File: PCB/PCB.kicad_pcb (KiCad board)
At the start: 2 copper layers, 53 parts, among them J1 USB_C_Receptacle_USB2.0_14P, Q1 IRLML2060, SW1 SW_Push, SW2 SW_Push, U1 RP2040, U2 W25Q16JVSS, U4 NCP1117-3.3_SOT223, U5 USBLC6-2SC6, Y1 Crystal_GND24

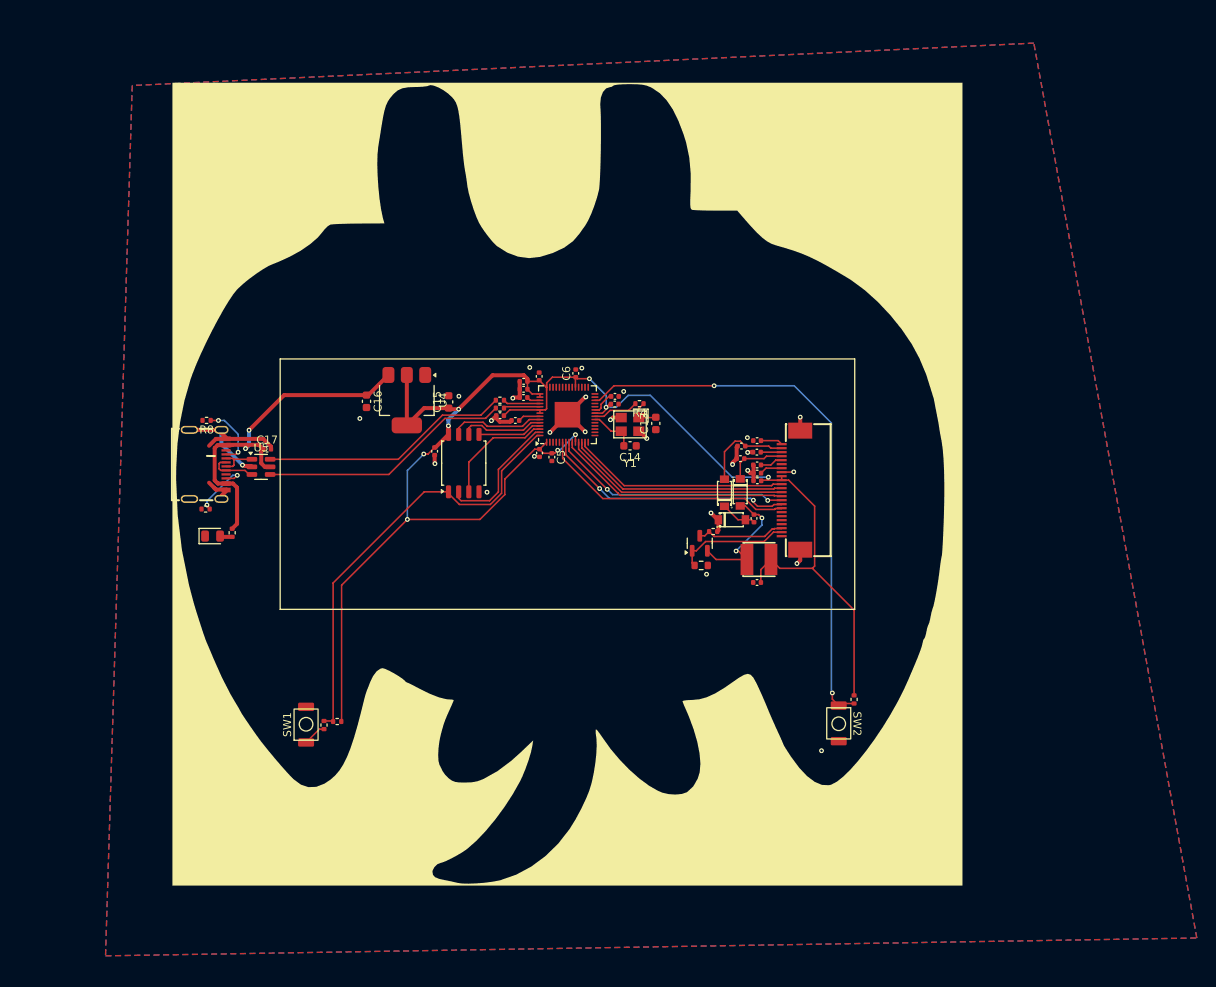
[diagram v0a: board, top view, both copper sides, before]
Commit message: commit beeg stuff(i forgor to commit for a while)
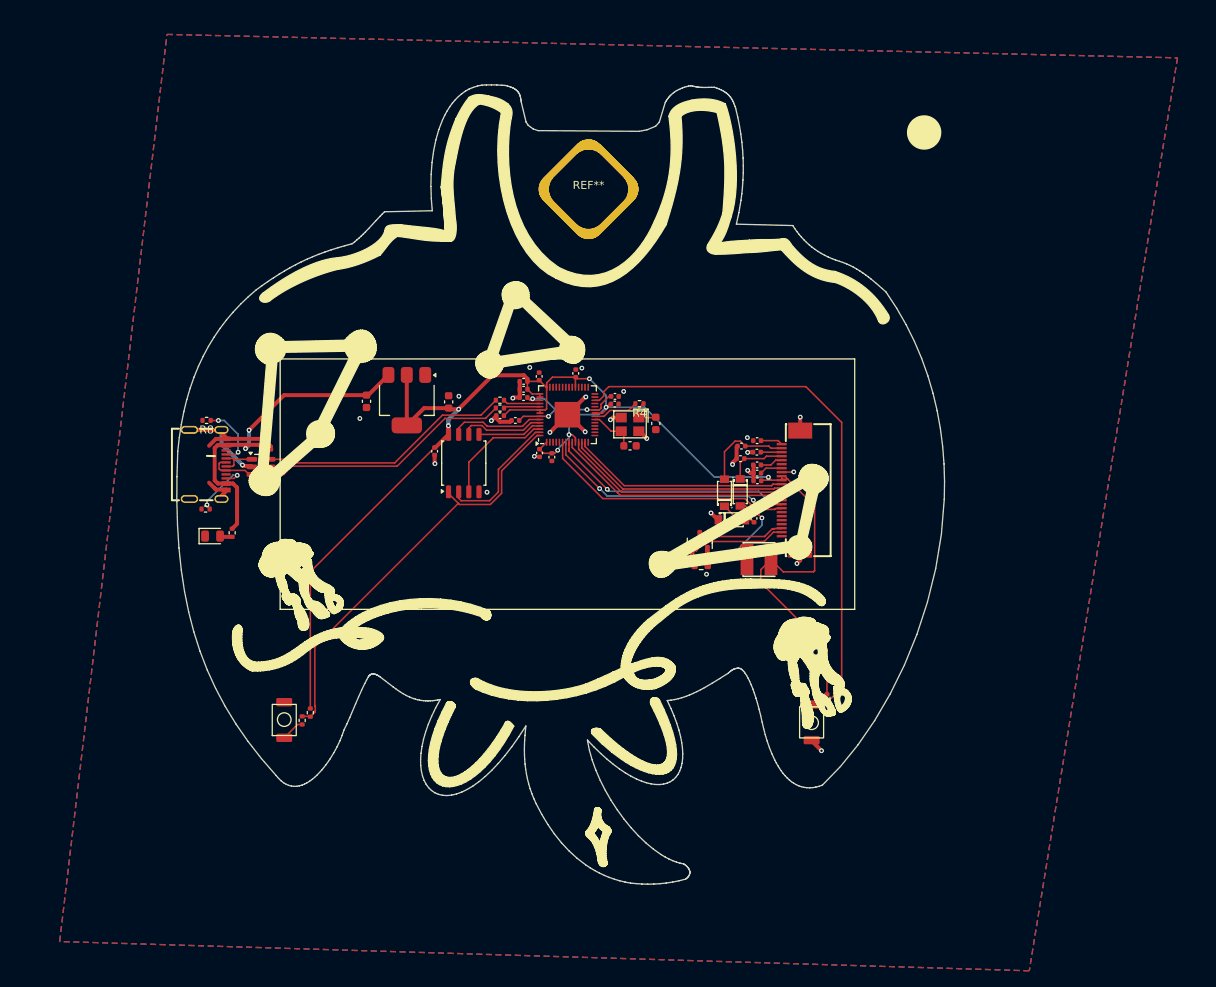
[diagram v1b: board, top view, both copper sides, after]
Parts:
- removed G***: LOGO, LOGO
- added REF**: Lanyard_hole2, Taranium-libs:Lanyard_hole2, F.Cu at (118.1, 34.1)
- moved R2 3.54 mm to (83.3, 99.6), turned to 90 degrees
- moved SW2 3.39 mm to (145.9, 100.8)
- moved R5 3.39 mm to (147.9, 97.8)
- moved R1 2.79 mm to (82.3, 100.5)
- moved SW1 2.79 mm to (80.0, 100.5)
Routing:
- net +3V3: track 198.6 -> 184.4 mm, vias 9 -> 7
- net +1V1: track 7.53 -> 18.4 mm, vias 0 -> 3
- net CS: track 55.1 -> 53.0 mm
- net GND: track 60.1 -> 61.9 mm
- net Net-(U1-RUN): track 70.0 -> 71.5 mm, vias 2 -> 0
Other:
- board outline added: 96 x 99.9 mm

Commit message: bleh
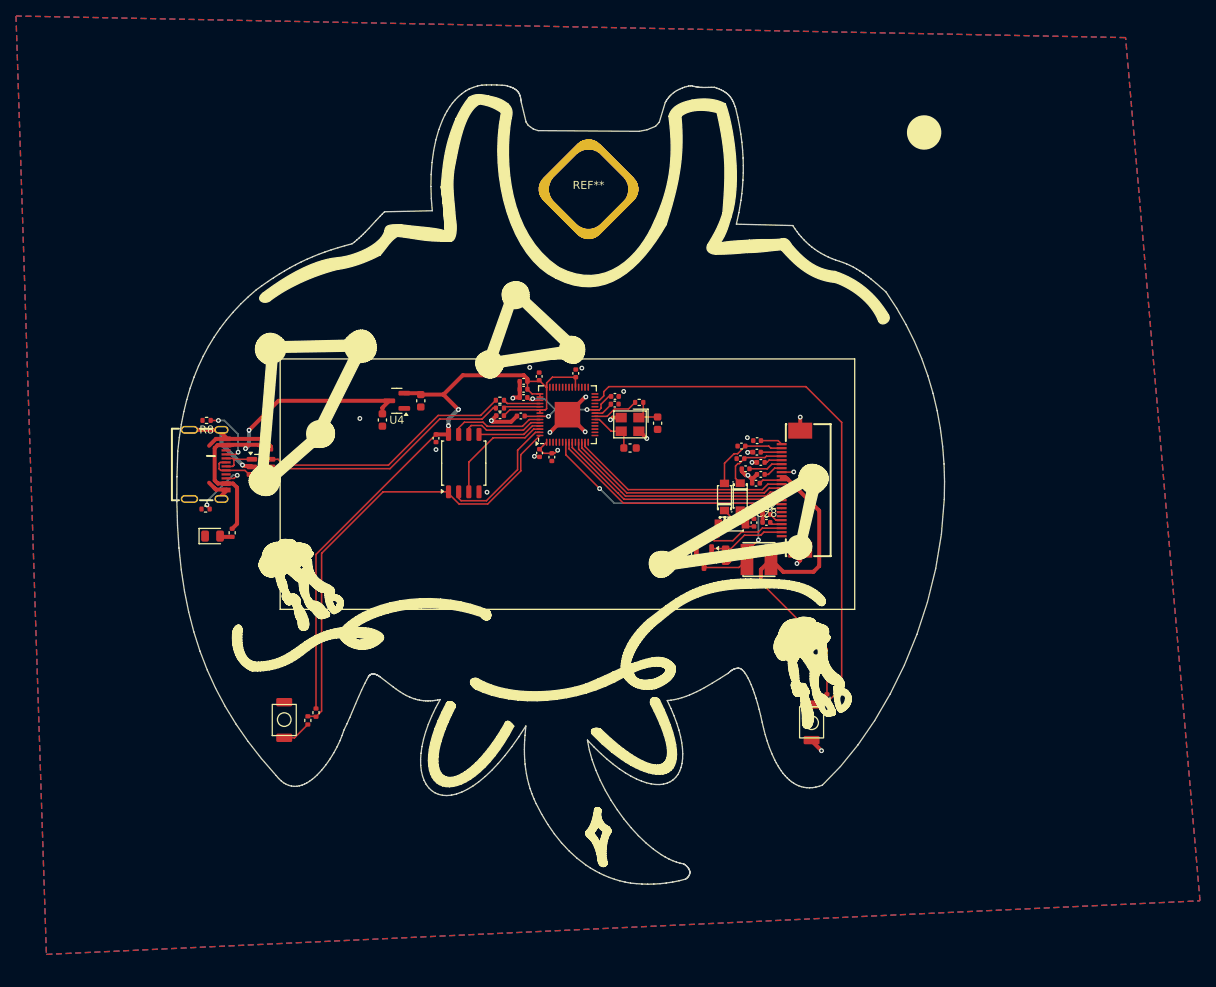
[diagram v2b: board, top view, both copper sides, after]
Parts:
- added C22: 1UF, Capacitor_SMD:C_0402_1005Metric, F.Cu at (140.3, 74.8)
- added C28: 1UF, Capacitor_SMD:C_0402_1005Metric, F.Cu at (140.3, 75.8)
- added C29: 1UF, Capacitor_SMD:C_0402_1005Metric, F.Cu at (137.7, 69.1)
- C21: value 1UF -> 100nf
- D2, D3, D4: value D_Small -> MBR0530
- L1: value L -> 10uh 1A
- R10: value 2.2 -> 0.47
- R11: value 1M -> 10k
- R6, R7: value 22 -> 90
- U4: value NCP1117-3.3_SOT223 -> XC6206P332MR; footprint Package_TO_SOT_SMD:SOT-223-3_TabPin2 -> Package_TO_SOT_SMD:SOT-23
- moved C15 3.49 mm to (97.1, 60.6), turned to -90 degrees
- moved R11 3.31 mm to (135.2, 79.9), turned to 90 degrees
- moved C16 3.07 mm to (92.3, 63.0)
- moved Q1 1.87 mm to (132.5, 80.2), turned to -90 degrees
- moved C12 1.64 mm to (99.0, 65.3)
- moved U4 1.26 mm to (94.1, 60.6), turned to 180 degrees
- moved C10 0.88 mm to (109.6, 62.5)
- moved R1 0.71 mm to (83.0, 100.5)
- moved R2 0.71 mm to (84.0, 99.6)
- moved C24 0.56 mm to (139.6, 68.3)
- moved C18 0.53 mm to (138.8, 75.8)
- moved D2 0.53 mm to (135.1, 72.6)
- moved D3 0.53 mm to (136.0, 76.0)
- moved D4 0.53 mm to (137.0, 72.6)
- moved R10 0.53 mm to (133.7, 77.5)
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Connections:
- net DM renamed DN
- net VCOM renamed /VCOM
- Q1 pad 2: Net-(D4-A) -> RESE
- Q1 pad 3: RESE -> Net-(D4-A)
- U1 pad 6: BS -> unconnected-(U1-GPIO4-Pad6)
- U3 pad 19: unconnected-(U3-VPP-Pad19) -> Net-(U3-VPP)
- U3 pad 4: unconnected-(U3-NC-Pad4) -> Net-(C28-Pad2)
- U3 pad 5: unconnected-(U3-VSH2-Pad5) -> Net-(U3-VSH2)
- U3 pad 8: BS -> GND
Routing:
- net +3V3: track 184.4 -> 138.2 mm, vias 7 -> 3
- net BS: track 32.1 -> 0.00 mm
- net CS: track 53.0 -> 57.7 mm
- net GDR: track 14.1 -> 9.69 mm
- net Net-(U3-VPP): track 0.00 -> 4.27 mm
- net Net-(U3-VSH2): track 0.00 -> 1.73 mm
- net Net-(C28-Pad2): track 0.00 -> 1.52 mm
- net RESE: track 11.7 -> 12.9 mm
- net VGH: track 7.54 -> 8.67 mm
- net Net-(D4-A): track 16.0 -> 17.0 mm
- net +1V1: track 18.4 -> 17.5 mm
- net VGL: track 11.5 -> 10.7 mm
- net +5V: track 46.1 -> 46.9 mm
- net Net-(R1-Pad1): track 2.93 -> 3.64 mm
- net Net-(U3-VSH1): track 2.84 -> 2.25 mm
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
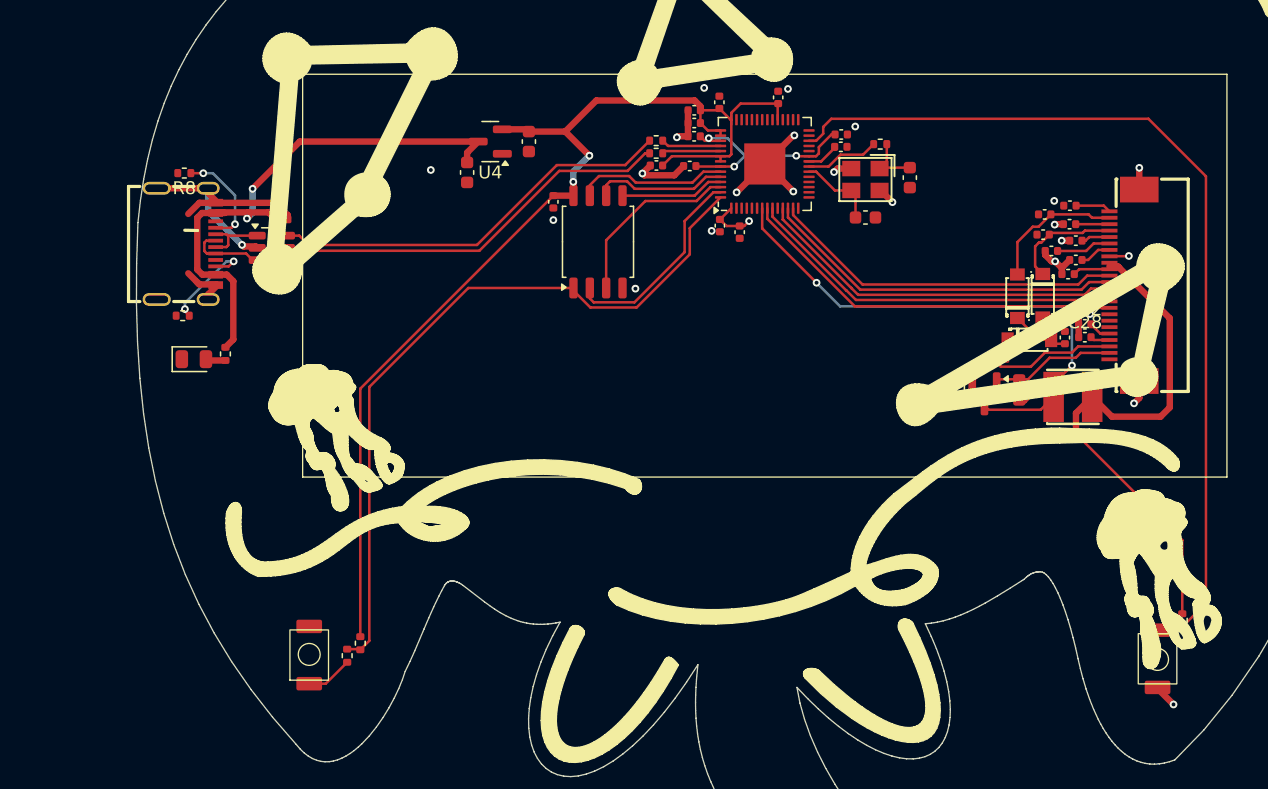
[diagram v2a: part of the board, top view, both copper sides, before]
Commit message: push
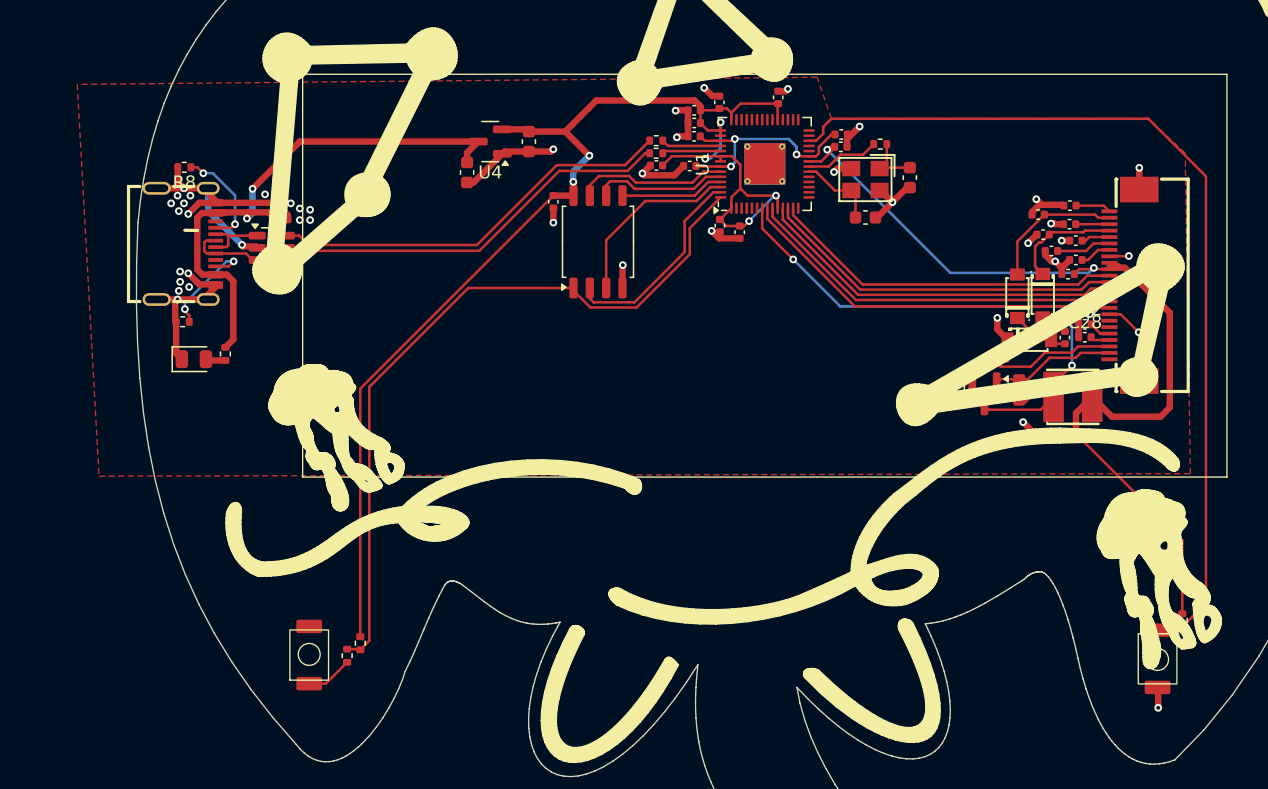
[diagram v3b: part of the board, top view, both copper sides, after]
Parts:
- U1: footprint Package_DFN_QFN:QFN-56-1EP_7x7mm_P0.4mm_EP3.2x3.2mm -> Package_DFN_QFN:QFN-56-1EP_7x7mm_P0.4mm_EP3.2x3.2mm_ThermalVias
- moved C26 0.51 mm to (136.7, 66.3)
- moved R9 0.47 mm to (70.2, 74.6)
- moved R8 0.45 mm to (70.3, 62.6)
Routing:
- net +3V3: track 138.2 -> 176.8 mm, vias 3 -> 8
- net GND: track 61.9 -> 99.8 mm, vias 23 -> 45
- net (no net): track 0.07 -> 0.00 mm, vias 2 -> 0
- added copper zone on F.Cu, net +3V3

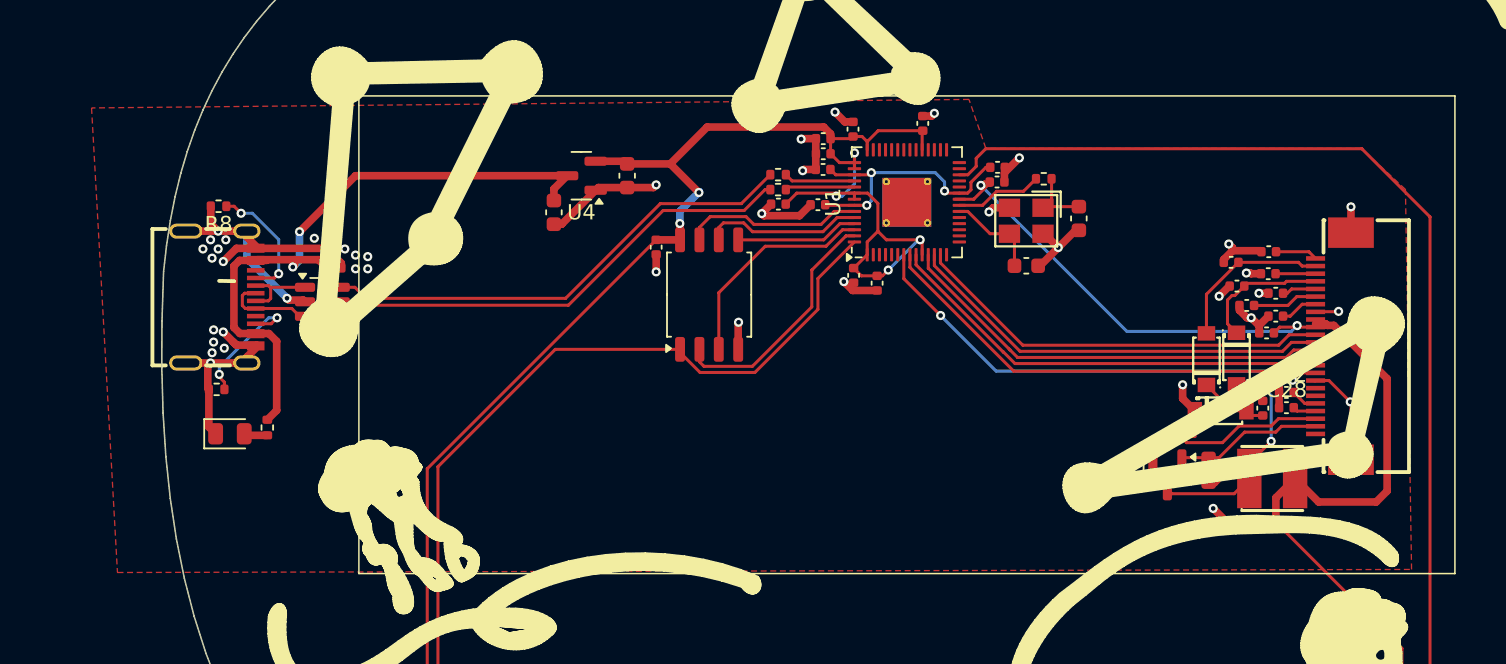
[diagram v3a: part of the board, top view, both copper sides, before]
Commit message: commit
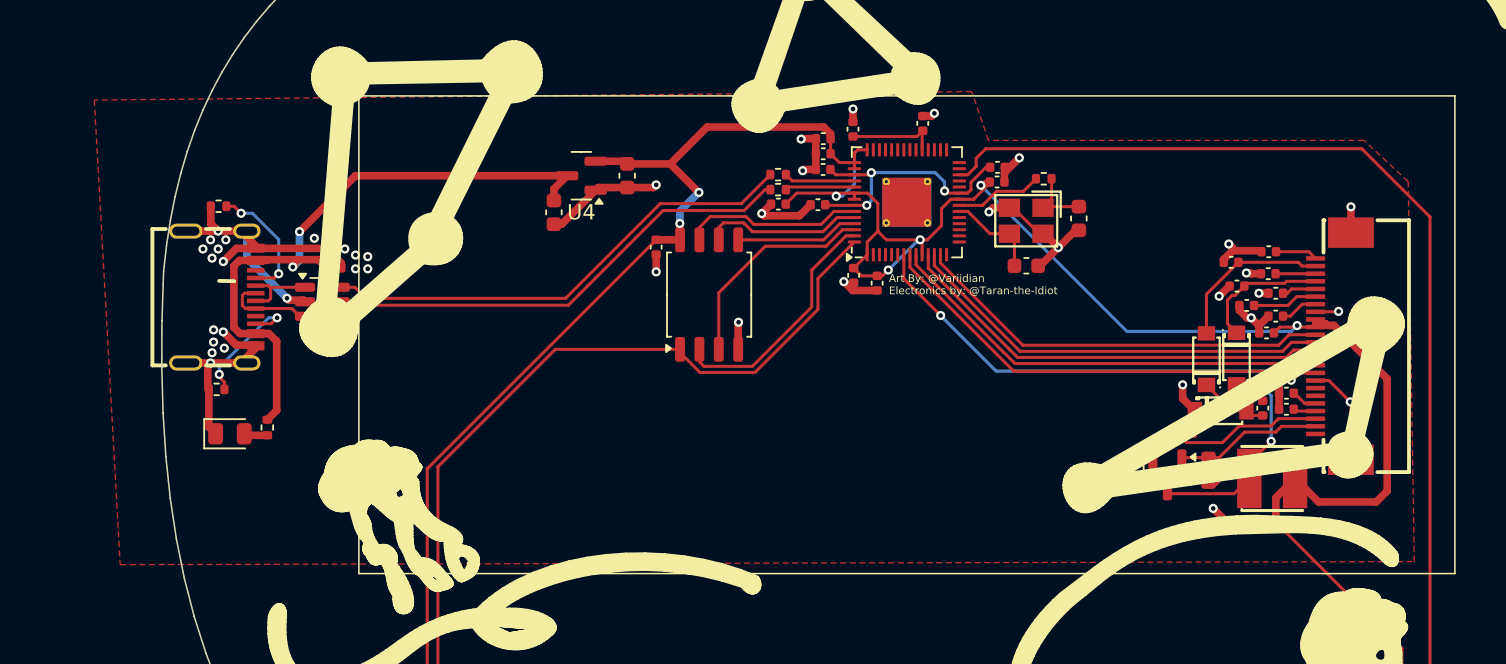
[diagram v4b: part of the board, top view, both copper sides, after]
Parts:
- moved C11 11.4 mm to (121.4, 60.0), turned to 0 degrees
- moved C9 11.4 mm to (109.9, 60.2), turned to 180 degrees
- moved C1 4.42 mm to (110.0, 59.2)
- moved C2 4.42 mm to (107.0, 62.5)
- moved C28 0.10 mm to (140.3, 75.9)
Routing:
- net +3V3: track 176.8 -> 180.0 mm, vias 8 -> 7
- net GND: track 99.8 -> 101.3 mm
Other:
- board text added: "Art By: @Variidian Electronics by: @Taran-the-Idiot"
